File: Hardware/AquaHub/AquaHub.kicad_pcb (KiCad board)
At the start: 2 copper layers, 170.2 x 116.2 mm, 62 parts, among them J1 Screw_Terminal_01x13, J10 PinHeader4, J11 Conn_01x06, J12 Conn_01x06, J13 Conn_01x02, J2 Screw_Terminal_01x13, J3 Screw_Terminal_01x13, J4 Screw_Terminal_01x13, J5 Screw_Terminal_01x13, J6 Screw_Terminal_01x13, J7 Screw_Terminal_01x13, J8 Screw_Terminal, J9 PinHeader3, K1 MT2-C93402, K2 MT2-C93402, K3 MT2-C93402, K4 MT2-C93402, K5 MT2-C93402, K6 MT2-C93402, SW1 SW_Push, SW2 SW_Push, SW3 SW_Push, SW4 SW_Push, SW5 SW_Push, SW6 SW_Push, U1 ESP32-WROOM, U2 MLX91210KDC-CAS-102-SP, U3 NCP1117DT33G, U4 TPL7407LA, U5 NCP1117DT50G, U6 TCA9534

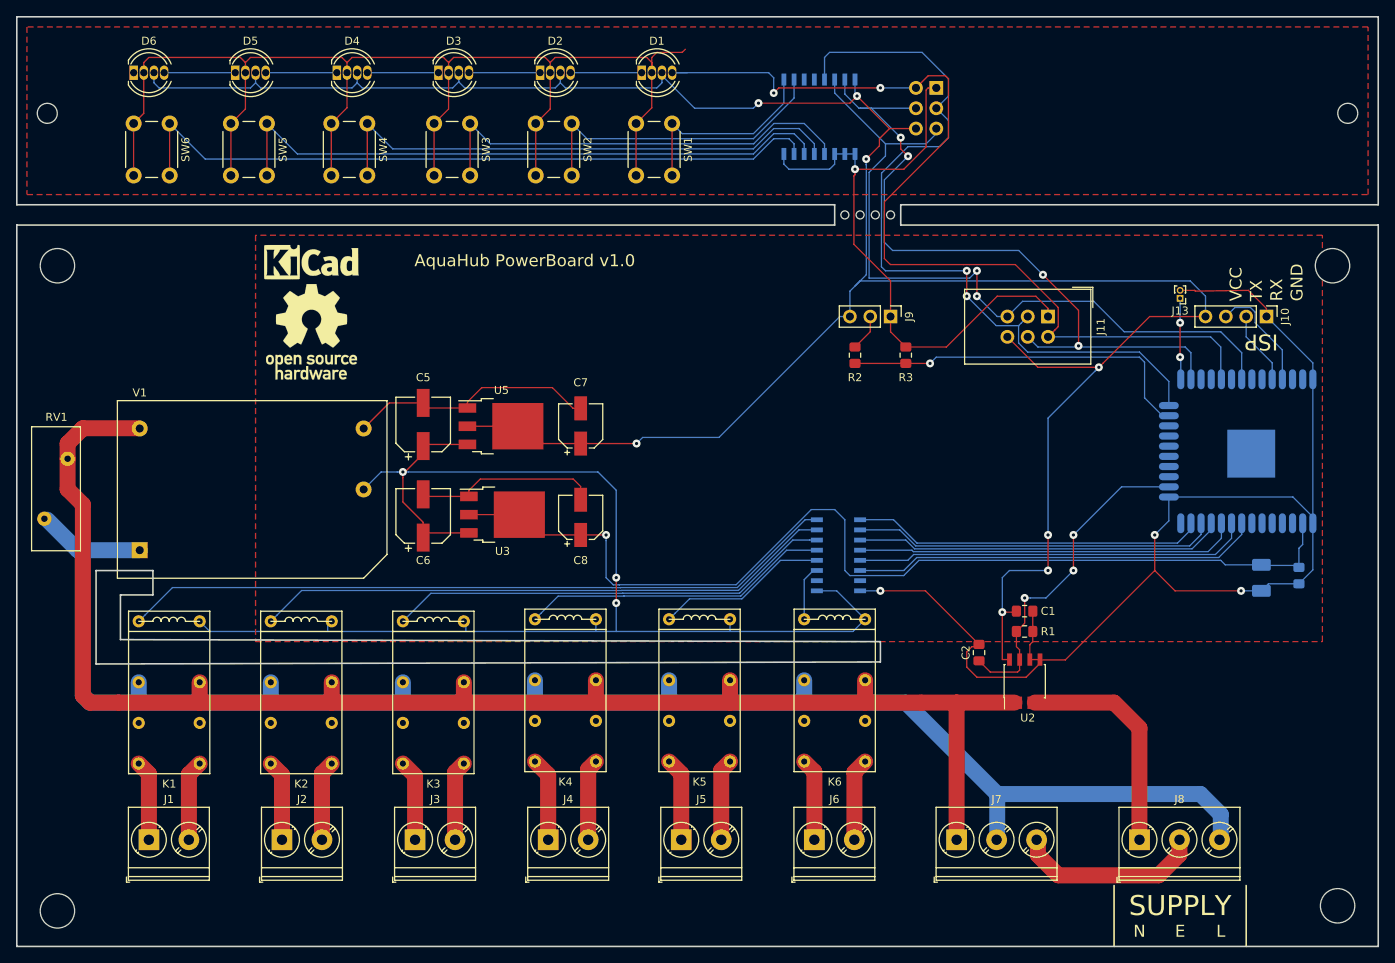
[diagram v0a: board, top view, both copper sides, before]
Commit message: Many refinements
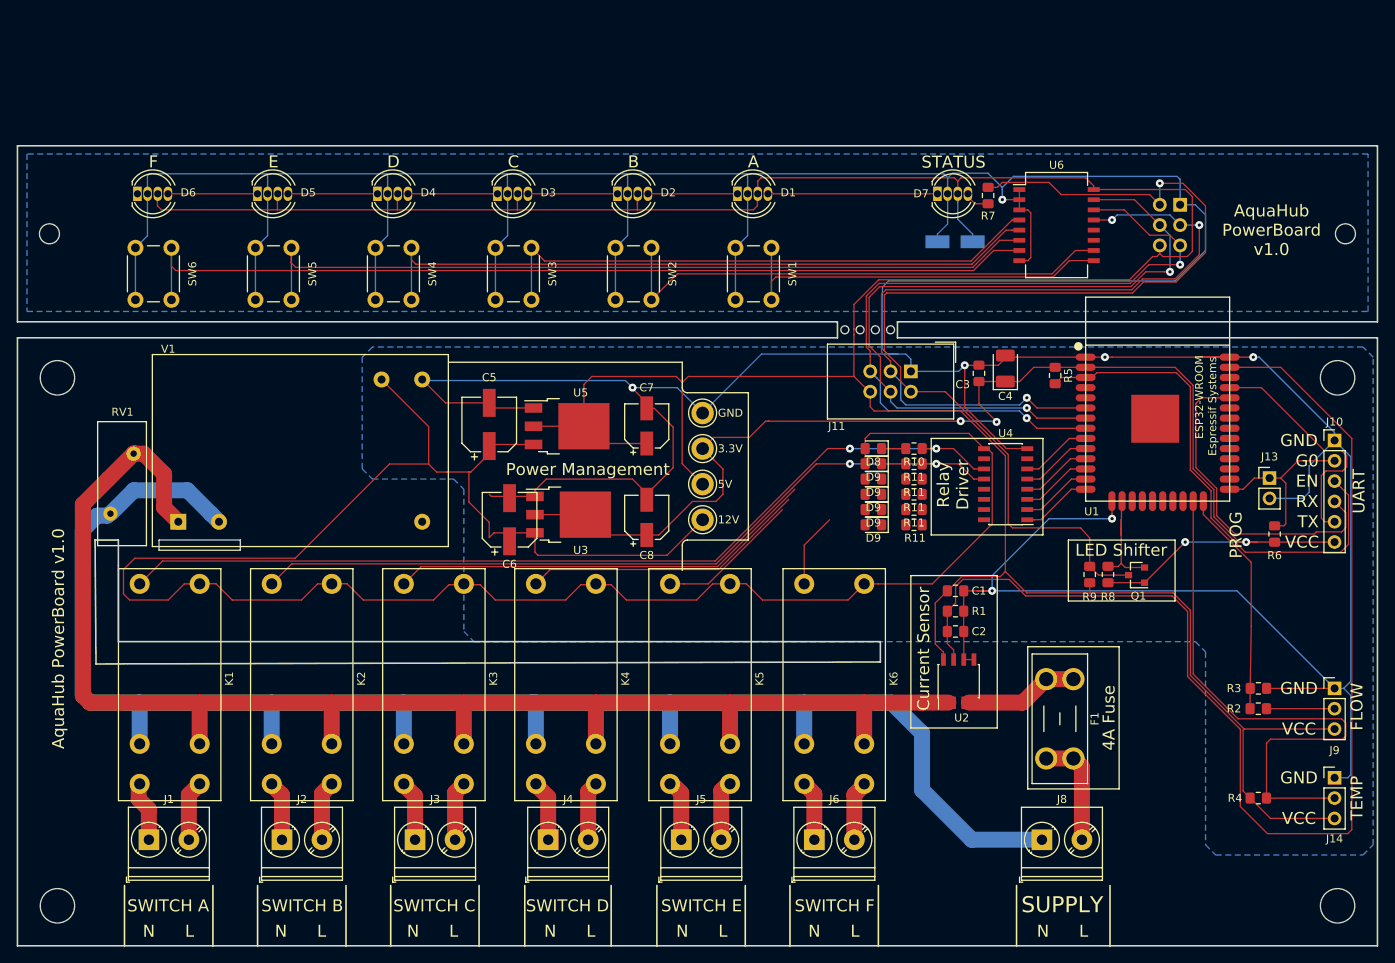
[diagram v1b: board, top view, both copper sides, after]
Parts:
- removed J7: Screw_Terminal_01x13, TerminalBlock_Phoenix:TerminalBlock_Phoenix_PT-1,5-3-5.0-H_1x03_P5.00mm_Horizontal
- removed REF**: OSHW-Logo_11.4x12mm_SilkScreen, Symbol:OSHW-Logo_11.4x12mm_SilkScreen
- removed REF**: KiCAD Logo, Symbol:Symbol_KiCAD-Logo_CopperAndSilkScreenTop
- added C9: 1000uF, Capacitor_SMD:CP_Elec_5x4.4, B.Cu at (155.4, 65.6)
- added D7: WS2811, LED_THT:LED_D5.0mm-4_RGB, F.Cu at (153.2, 59.6)
- added D8: Green, LED_SMD:LED_0805_2012Metric_Pad1.15x1.40mm_HandSolder, F.Cu at (145.2, 91.4)
- added D9: Green, LED_SMD:LED_0805_2012Metric_Pad1.15x1.40mm_HandSolder, F.Cu at (145.2, 101.0)
- added D9: Green, LED_SMD:LED_0805_2012Metric_Pad1.15x1.40mm_HandSolder, F.Cu at (145.2, 99.1)
- added D9: Green, LED_SMD:LED_0805_2012Metric_Pad1.15x1.40mm_HandSolder, F.Cu at (145.2, 97.2)
- added D9: Green, LED_SMD:LED_0805_2012Metric_Pad1.15x1.40mm_HandSolder, F.Cu at (145.2, 95.2)
- added D9: Green, LED_SMD:LED_0805_2012Metric_Pad1.15x1.40mm_HandSolder, F.Cu at (145.2, 93.3)
- added F1: 4A, Fuse:Fuseholder_Blade_Mini_Keystone_3568, F.Cu at (170.2, 120.3)
- added J14: PinHeader3, Connector_PinHeader_2.54mm:PinHeader_1x03_P2.54mm_Vertical, F.Cu at (202.8, 132.6)
- added Q1: BSS138, Package_TO_SOT_SMD:SOT-23, F.Cu at (178.1, 107.3)
- added R10: 680R, Resistor_SMD:R_0805_2012Metric_Pad1.15x1.40mm_HandSolder, F.Cu at (150.2, 91.4)
- added R11: 680R, Resistor_SMD:R_0805_2012Metric_Pad1.15x1.40mm_HandSolder, F.Cu at (150.2, 101.0)
- added R11: 680R, Resistor_SMD:R_0805_2012Metric_Pad1.15x1.40mm_HandSolder, F.Cu at (150.2, 99.1)
- added R11: 680R, Resistor_SMD:R_0805_2012Metric_Pad1.15x1.40mm_HandSolder, F.Cu at (150.2, 97.2)
- added R11: 680R, Resistor_SMD:R_0805_2012Metric_Pad1.15x1.40mm_HandSolder, F.Cu at (150.2, 95.2)
- added R11: 680R, Resistor_SMD:R_0805_2012Metric_Pad1.15x1.40mm_HandSolder, F.Cu at (150.2, 93.3)
- added R4: 4.7K, Resistor_SMD:R_0805_2012Metric_Pad1.15x1.40mm_HandSolder, F.Cu at (193.3, 135.1)
- added R5: 10k, Resistor_SMD:R_0805_2012Metric_Pad1.15x1.40mm_HandSolder, F.Cu at (167.9, 82.3)
- added R6: 10k, Resistor_SMD:R_0805_2012Metric_Pad1.15x1.40mm_HandSolder, F.Cu at (195.3, 102.1)
- added R7: 500R, Resistor_SMD:R_0805_2012Metric_Pad1.15x1.40mm_HandSolder, F.Cu at (159.5, 59.8)
- added R8: 10k, Resistor_SMD:R_0805_2012Metric_Pad1.15x1.40mm_HandSolder, F.Cu at (174.5, 107.2)
- added R9: 10k, Resistor_SMD:R_0805_2012Metric_Pad1.15x1.40mm_HandSolder, F.Cu at (172.2, 107.2)
- added TP1: TestPoint, TestPoint:TestPoint_Keystone_5010-5014_Multipurpose, F.Cu at (123.8, 95.9)
- added TP2: TestPoint, TestPoint:TestPoint_Keystone_5010-5014_Multipurpose, F.Cu at (123.8, 91.4)
- added TP3: TestPoint, TestPoint:TestPoint_Keystone_5010-5014_Multipurpose, F.Cu at (123.8, 87.0)
- added TP4: TestPoint, TestPoint:TestPoint_Keystone_5010-5014_Multipurpose, F.Cu at (123.8, 100.3)
- C3, C4, U1, U4, U6: moved to F.Cu
- D1, D2, D3, D4, D5, D6: value NeoPixel -> WS2811
- J1, J2, J3, J4, J5, J6: value Screw_Terminal_01x13 -> Screw_Terminal_01x02
- J10: value PinHeader4 -> PinHeader6; footprint Connector_PinHeader_2.54mm:PinHeader_1x04_P2.54mm_Vertical -> Connector_PinHeader_2.54mm:PinHeader_1x06_P2.54mm_Vertical
- J11, J12: value Conn_01x06 -> IDC_2x3
- J13: value Conn_01x02 -> PinHeader2; footprint Connector_PinHeader_1.00mm:PinHeader_1x02_P1.00mm_Vertical -> Connector_PinHeader_2.54mm:PinHeader_1x02_P2.54mm_Vertical
- J8: value Screw_Terminal -> Screw_Terminal_01x02; footprint TerminalBlock_Phoenix:TerminalBlock_Phoenix_PT-1,5-3-5.0-H_1x03_P5.00mm_Horizontal -> TerminalBlock_Phoenix:TerminalBlock_Phoenix_PT-1,5-2-5.0-H_1x02_P5.00mm_Horizontal
- K1, K2, K3, K4, K5, K6: value MT2-C93402 -> FTR-F1AA012V; footprint AquaFootprints:MT2-C93400 -> AquaFootprints:fujitsu-ftr1-a
- R1: value 6k-100k? -> 10k
- V1: value RAC01-12SGB -> RAC04-12SGB; footprint Converter_ACDC:Converter_ACDC_RECOM_RAC01-xxSGB_THT -> Converter_ACDC:Converter_ACDC_RECOM_RAC04-xxSGB_THT
- moved J9 72.4 mm to (202.8, 121.4), turned to 0 degrees
- moved R2 67.0 mm to (193.3, 124.0), turned to 0 degrees
- moved R3 60.6 mm to (193.3, 121.4), turned to 180 degrees
- moved C3 47.3 mm to (158.4, 82.0), turned to 90 degrees
- moved C4 41.3 mm to (161.7, 81.4), turned to 90 degrees
- moved J12 33.8 mm to (183.5, 61.0)
- moved U6 32.6 mm to (168.1, 63.5), turned to 0 degrees
- moved J13 25.1 mm to (194.7, 95.1), turned to 0 degrees
- moved U4 22.7 mm to (161.7, 95.9)
- moved K5 21.9 mm to (127.3, 133.3), turned to 90 degrees
- moved K4 21.9 mm to (110.5, 133.3), turned to 90 degrees
- moved K6 21.9 mm to (144.0, 133.3), turned to 90 degrees
- moved K2 21.7 mm to (77.5, 133.3), turned to 90 degrees
- moved K3 21.7 mm to (94.0, 133.3), turned to 90 degrees
- moved K1 21.7 mm to (61.0, 133.3), turned to 90 degrees
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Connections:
- net NEUTRAL1 renamed /NEUTRAL1
- net NEUTRAL2 renamed /NEUTRAL2
- net NEUTRAL3 renamed /NEUTRAL3
- net NEUTRAL4 renamed /NEUTRAL4
- net NEUTRAL5 renamed /NEUTRAL5
- net NEUTRAL6 renamed /NEUTRAL6
- C1 pad 1: +5V -> GND
- C1 pad 2: GND -> +5V
- D1 pad 4: /Panel_LED -> Net-(D1-Pad4)
- J1 pad 2: LIVE1 -> /LIVE1
- J10 pad 2: /RX -> /G0
- J10 pad 3: /TX -> /EN
- J10 pad 4: +5V -> /RX
- J13 pad 1: Net-(J13-Pad1) -> /G0
- J2 pad 2: LIVE2 -> /LIVE2
- J3 pad 2: LIVE3 -> /LIVE3
- J4 pad 2: LIVE4 -> /LIVE4
- J5 pad 2: LIVE5 -> /LIVE5
- J6 pad 2: LIVE6 -> /LIVE6
- J8 pad 1: /LIVE_IN -> /NEUTRAL
- J8 pad 2: EARTH -> /UNFUSED_LIVE
- K1 pad 1: RE1 -> /LIVE1
- K1 pad 4: NEUTRAL -> +12V
- K2 pad 1: RE2 -> /LIVE2
- K2 pad 4: NEUTRAL -> +12V
- K3 pad 1: RE3 -> /LIVE3
- K3 pad 4: NEUTRAL -> +12V
- K4 pad 1: RE4 -> /LIVE4
- K4 pad 4: NEUTRAL -> +12V
- K5 pad 1: RE5 -> /LIVE5
- K5 pad 4: NEUTRAL -> +12V
- K6 pad 1: RE6 -> /LIVE6
- K6 pad 4: NEUTRAL -> +12V
- R2 pad 1: /FLOW_SENSE -> /Flow_Sense
- R3 pad 2: /FLOW_SENSE -> /Flow_Sense
- RV1 pad 1: LIVE -> /LIVE
- RV1 pad 2: NEUTRAL -> /NEUTRAL
- U1 pad 10: /POW4 -> /POW2
- U1 pad 12: /POW2 -> /POW4
- U1 pad 13: /POW1 -> /POW5
- U1 pad 14: (no net) -> /POW6
- U1 pad 16: /Power_Sense -> /Panel_LED_33
- U1 pad 23: /FLOW_SENSE -> /Temp_Sense
- U1 pad 24: /Panel_INT -> /Flow_Sense
- U1 pad 25: Net-(J13-Pad1) -> /G0
- U1 pad 26: /Panel_SDA -> (no net)
- U1 pad 29: /Panel_LED -> (no net)
- U1 pad 3: (no net) -> /EN
- U1 pad 31: /Panel_SCL -> (no net)
- U1 pad 37: (no net) -> /Power_Sense
- U1 pad 6: (no net) -> /Panel_INT
- U1 pad 7: (no net) -> /Panel_SDA
- U1 pad 8: /POW6 -> /Panel_SCL
- U1 pad 9: /POW5 -> /POW1
- U2 pad 1: LIVE -> /LIVE
- U2 pad 2: LIVE -> /LIVE
- U4 pad 1: /POW1 -> /POW6
- U4 pad 11: RE6 -> /RE1
- U4 pad 12: RE5 -> /RE2
- U4 pad 13: RE4 -> /RE3
- U4 pad 14: RE3 -> /RE4
- U4 pad 15: RE2 -> /RE5
- U4 pad 16: RE1 -> /RE6
- U4 pad 2: /POW2 -> /POW5
- U4 pad 3: /POW3 -> /POW4
- U4 pad 4: /POW4 -> /POW3
- U4 pad 5: /POW5 -> /POW2
- U4 pad 6: /POW6 -> /POW1
- V1 pad 1: NEUTRAL -> /LIVE
- V1 pad 2: LIVE -> /NEUTRAL
- V1 pad 3: GND -> (no net)
- V1 pad 4: +12V -> GND
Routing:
- net GND: track 453.8 -> 671.0 mm, vias 4 -> 7
- net /NEUTRAL: track 0.00 -> 206.0 mm
- net NEUTRAL: track 205.1 -> 0.00 mm
- net LIVE: track 193.3 -> 0.00 mm
- net /LIVE: track 0.00 -> 185.6 mm
- net /RE1: track 0.00 -> 115.8 mm, vias 0 -> 2
- net /Power_Sense: track 41.8 -> 151.4 mm, vias 3 -> 0
- net +5V: track 316.7 -> 415.5 mm, vias 8 -> 0
- net /RE2: track 0.00 -> 98.2 mm, vias 0 -> 2
- net +12V: track 174.3 -> 266.2 mm, vias 3 -> 0
- net RE1: track 90.0 -> 0.00 mm
- net RE2: track 73.0 -> 0.00 mm
- net /Temp_Sense: track 0.00 -> 70.5 mm
- net /EN: track 0.00 -> 63.7 mm
- net RE3: track 56.2 -> 0.00 mm
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- added copper zone on B.Cu, net GND
- removed copper zone on F.Cu, net GND
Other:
- board size 170.2 x 116.2 mm -> 170 x 100 mm
- board text added: "12V"
- board text added: "3.3V"
- board text added: "4A Fuse"
- board text added: "5V"
- board text added: "A"
- board text added: "B"
- board text added: "C"
- board text added: "Current Sensor"
- board text added: "D"
- board text added: "EN"
- board text added: "F"
- board text added: "FLOW"
- board text added: "G0"
- board text added: "LED Shifter"
- board text added: "Mechanical parts must be on a metric grid."
- board text added: "PROG"
- board text added: "Power Management"
- board text added: "Relay Driver"
- board text added: "STATUS"
- board text added: "SWITCH A"
- board text added: "SWITCH B"
- board text added: "SWITCH C"
- board text added: "SWITCH D"
- board text added: "SWITCH E"
- board text added: "SWITCH F"
- board text added: "TEMP"
- board text added: "UART"
- board text removed: "ISP"
